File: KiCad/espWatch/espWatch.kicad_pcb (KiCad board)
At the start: 2 copper layers, 96.5 x 79.4 mm, 8 parts, among them J1 2-pin_power_input_header, U2 NodeMCU_1.0_(ESP-12E), U3 1.8" TFT ST7735, U4 RTC DS3231, U5 KY-040_Rotary_Encoder

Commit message: new schematics for esp
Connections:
- net /SCL L renamed SCL RTC
- net /SDA L renamed SDA RTC
- net Net-(BZ1-Pad1) renamed BUZ
- net Net-(U2-Pad21) renamed SDA SCR
- net Net-(U2-Pad23) renamed SCL SCR
- net Net-(U2-Pad26) renamed DC
- net Net-(U2-Pad27) renamed CS
- net Net-(U2-Pad30) renamed SW
- net Net-(U2-Pad4) renamed CLK
- net Net-(U2-Pad5) renamed DT

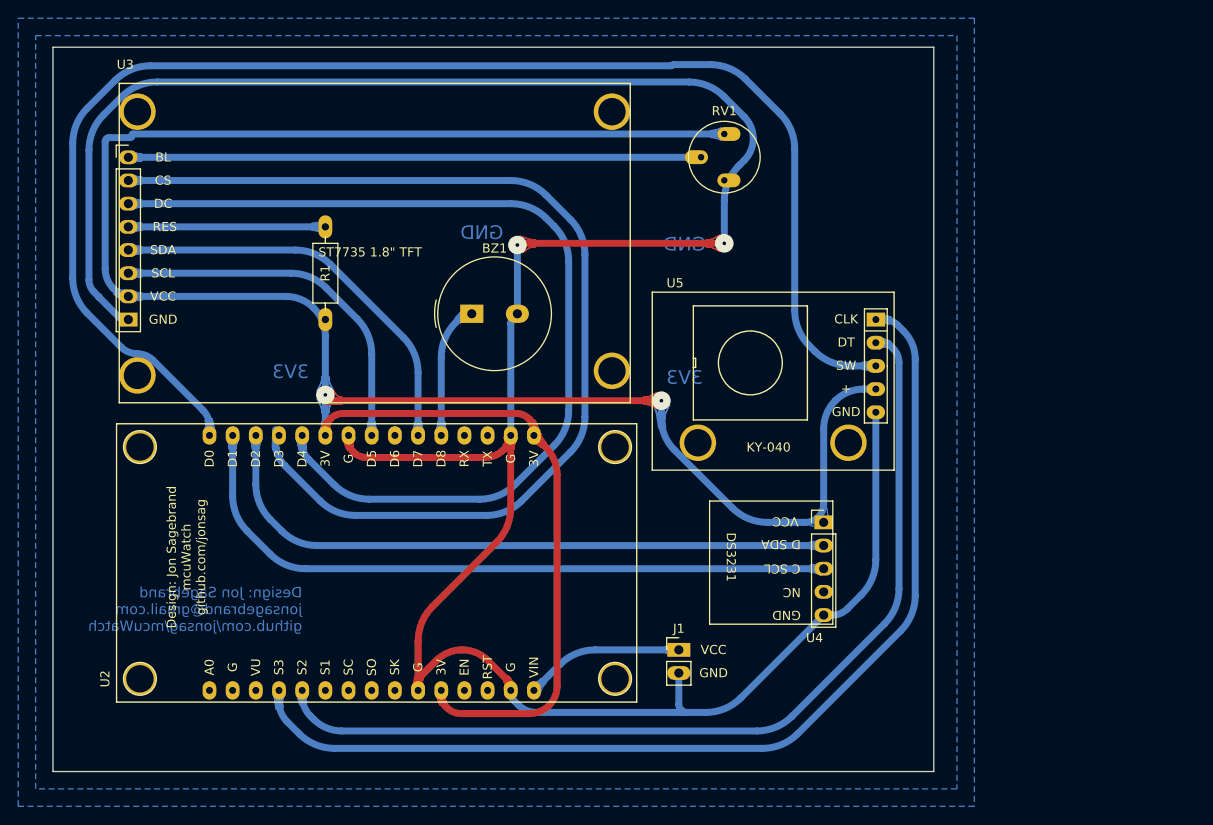
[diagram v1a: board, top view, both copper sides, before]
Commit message: new pcb
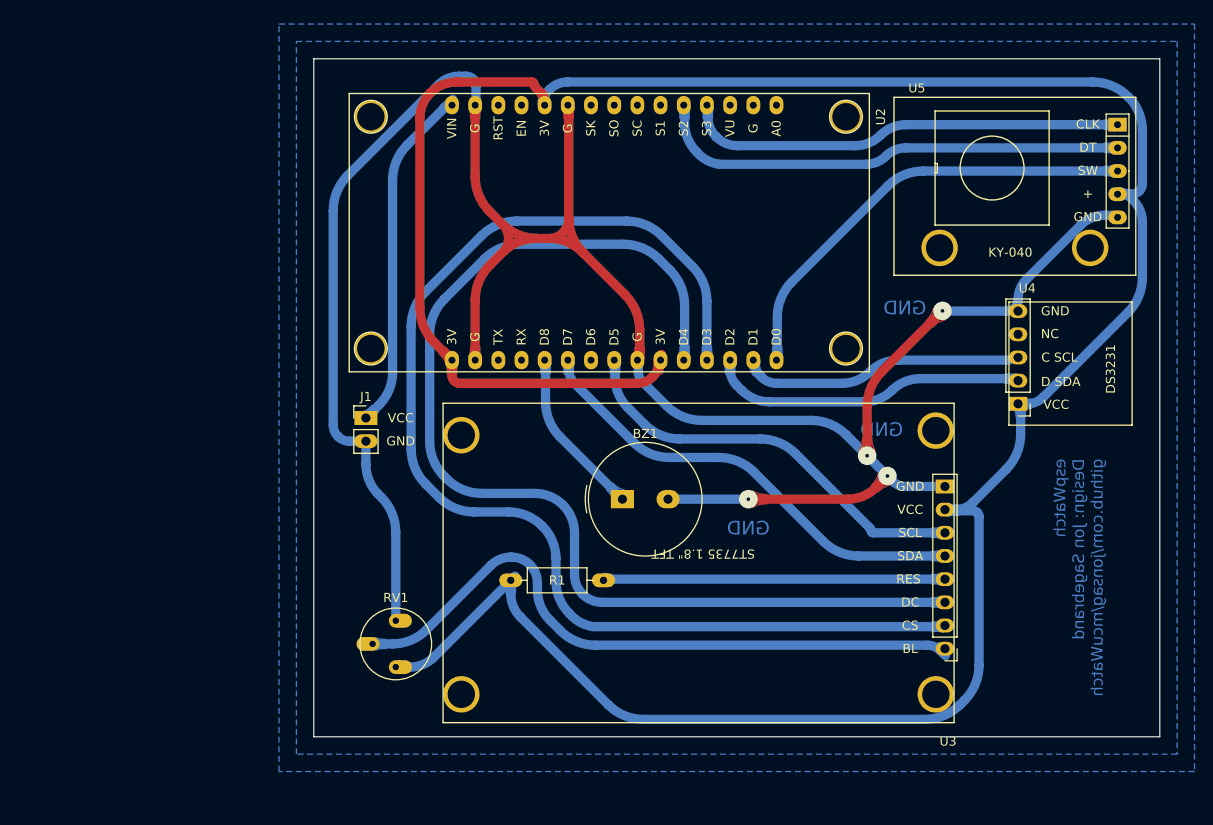
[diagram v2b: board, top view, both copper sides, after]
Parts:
- moved U3 104.4 mm to (169.5, 112.3), turned to 180 degrees
- moved U2 89.3 mm to (151.0, 52.7), turned to -90 degrees
- moved RV1 64.4 mm to (109.3, 114.3)
- moved J1 42.7 mm to (106.0, 87.0)
- moved U4 39.5 mm to (177.5, 75.3), turned to 0 degrees
- moved R1 35.1 mm to (121.9, 104.8), turned to 0 degrees
- moved U5 34.0 mm to (188.4, 54.8)
- moved BZ1 26.2 mm to (134.2, 95.9)
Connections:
- RV1 pad 1: GND -> +3V3
- RV1 pad 3: +3V3 -> GND
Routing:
- net SW: track 156.8 -> 49.4 mm
- net CLK: track 113.9 -> 48.5 mm
- net DT: track 104.5 -> 52.4 mm
- net SCL RTC: track 74.9 -> 30.1 mm
- net SDA RTC: track 71.2 -> 34.6 mm
- net GND: track 291.3 -> 259.1 mm, vias 2 -> 4
- net +3V3: track 272.7 -> 298.2 mm, vias 2 -> 0
- net +5V: track 17.5 -> 38.4 mm
- net Net-(R1-Pad2): track 21.6 -> 38.1 mm
- net CS: track 116.3 -> 132.7 mm
- net DC: track 105.7 -> 121.8 mm
- net Net-(RV1-Pad2): track 62.8 -> 72.2 mm
- net SCL SCR: track 39.4 -> 45.6 mm
- net SDA SCR: track 45.0 -> 50.3 mm
- net BUZ: track 15.0 -> 18.5 mm
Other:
- board size 96.5 x 79.4 mm -> 92.7 x 74.3 mm
- board text added: "espWatch Design: Jon Sagebrand github.com/jonsag/mcuWatch"
- board text removed: "3V3"
- board text removed: "Design: Jon Sagebrand jonsagebrand@gmail.com github.com/jonsag/mcuWatch"
- board text removed: "Design: Jon Sagebrand mcuWatch github.com/jonsag"
